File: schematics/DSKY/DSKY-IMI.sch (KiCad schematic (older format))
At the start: 7 parts, among them J103 Conn_02x08, J104 Conn_02x10, U19 74LS04, U42 74LS04, U46 74LS04, U5 74LS04, U6 74LS00

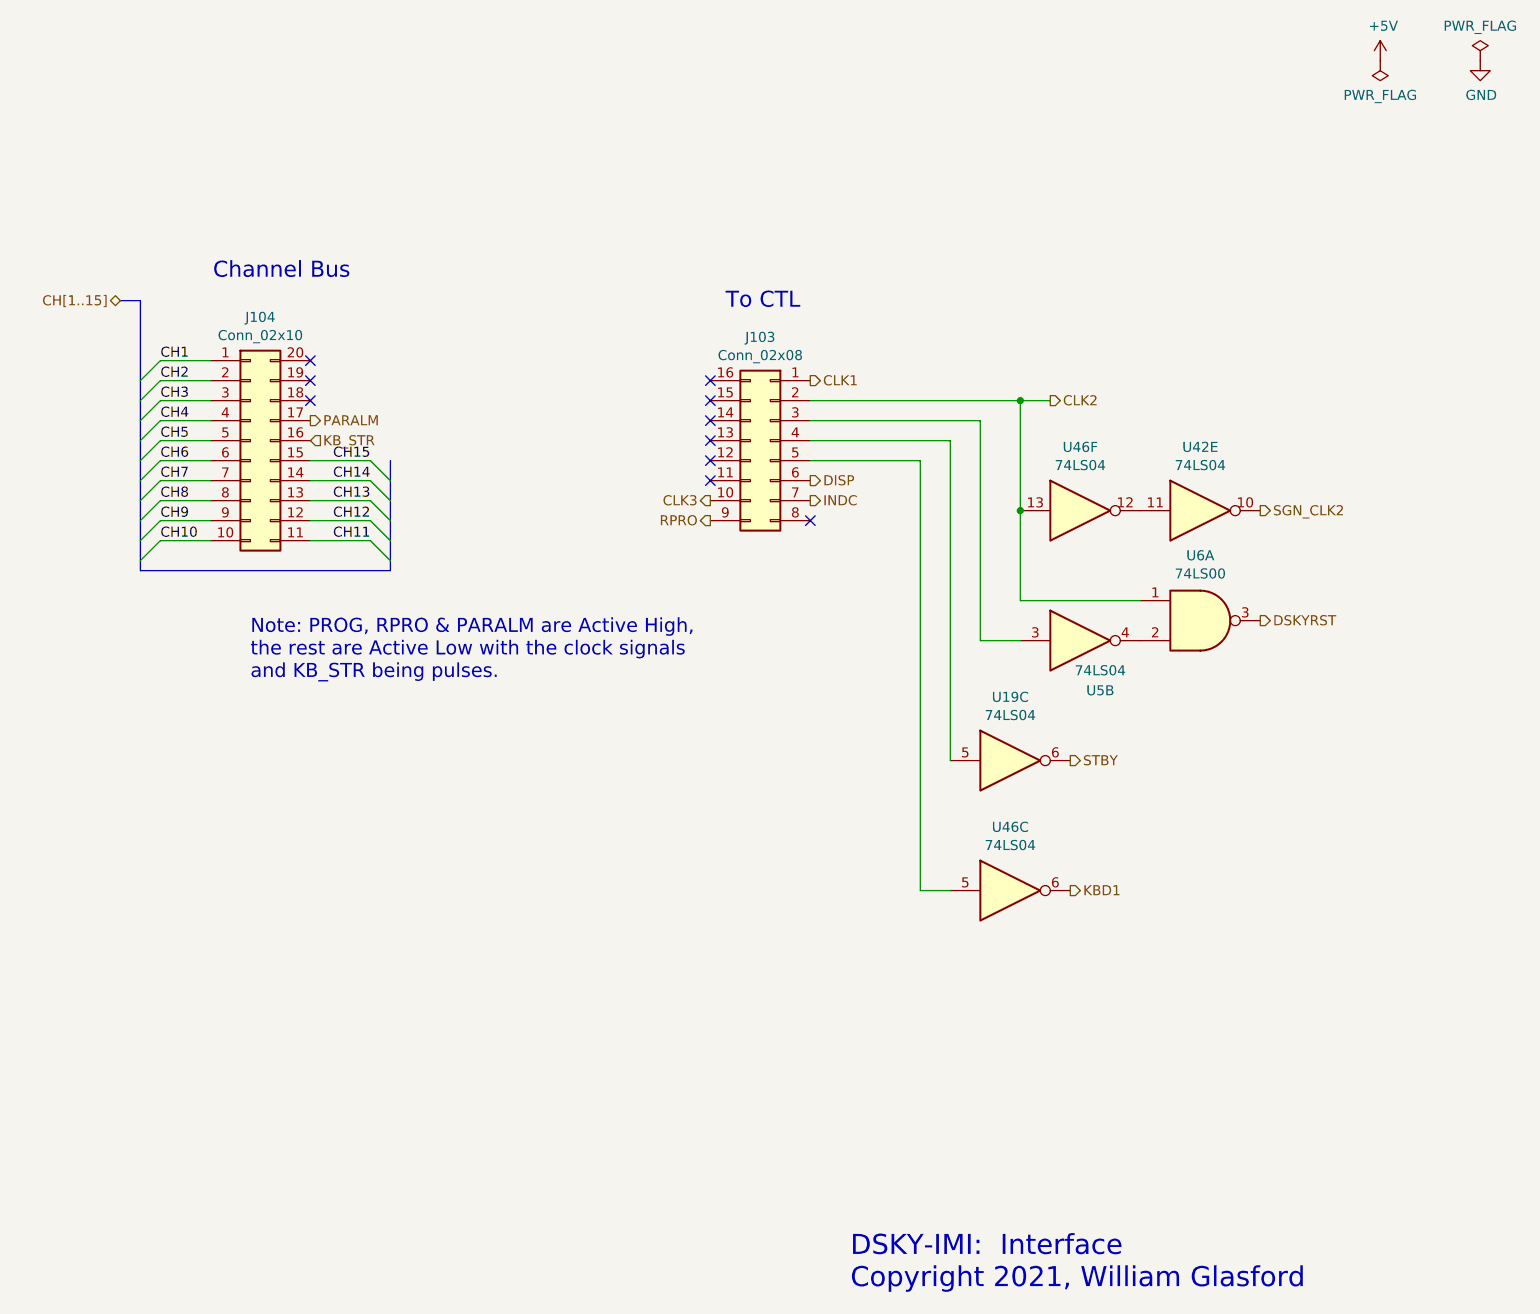
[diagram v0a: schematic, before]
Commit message: DSKY Redesign
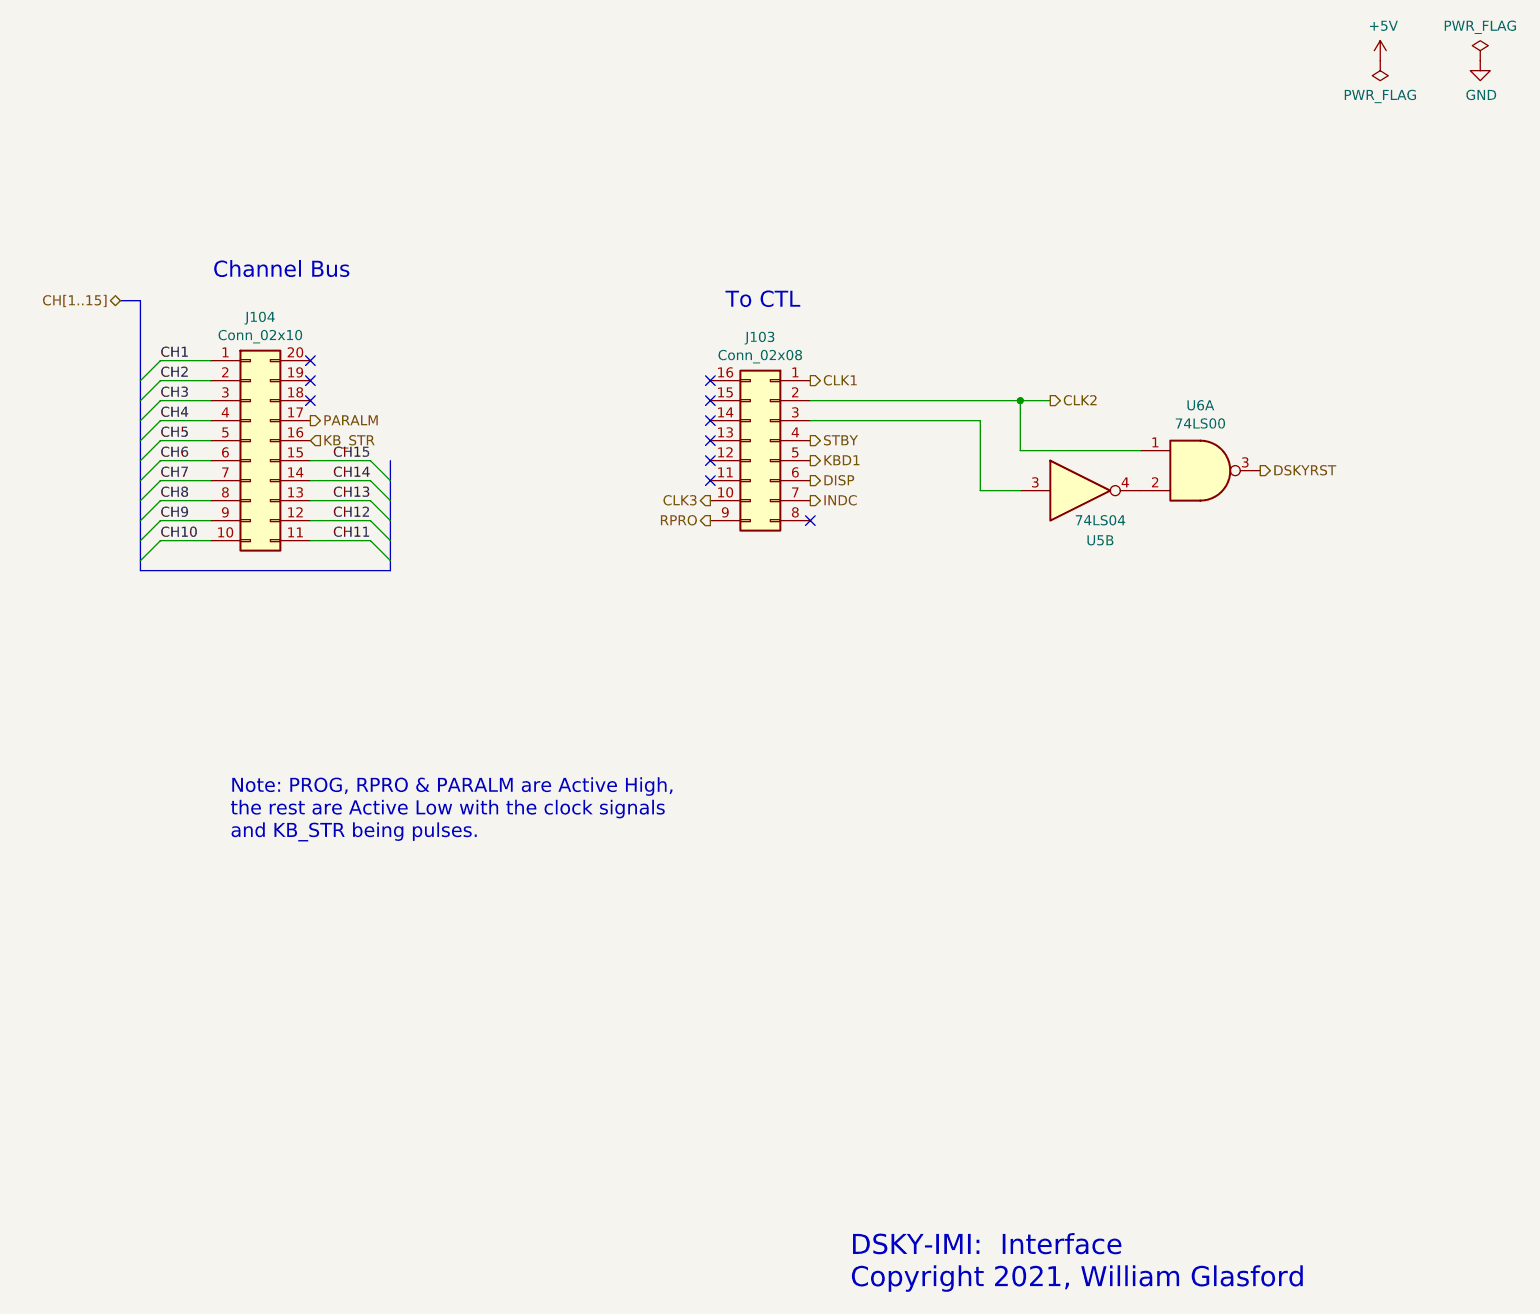
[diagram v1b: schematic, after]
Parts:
- removed U19, U42, U46: 74LS04, symbol 74xx:74LS04
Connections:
- net KBD1: now also J103.5 (Pin_5)
- net STBY: now also J103.4 (Pin_4)
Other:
- moved on the sheet: U5B, U6A
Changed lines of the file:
@@
 $Descr A 11000 8500
 encoding utf-8
-Sheet 10 12
+Sheet 2 15
 Title ""
 Date ""
@@
 Wire Wire Line
 	3750 3000 4050 3000
-Text HLabel 7550 4500 2    50   Output ~ 0
+Text HLabel 6250 2900 2    50   Output ~ 0
 STBY
 Text HLabel 3750 2900 2    50   Input ~ 0
@@
 Text Notes 6200 2250 2    80   ~ 0
 To CTL
-Text HLabel 7550 5150 2    50   Output ~ 0
+Text HLabel 6250 3000 2    50   Output ~ 0
 KBD1
 Text HLabel 6250 3100 2    50   Output ~ 0
@@
 Text HLabel 6250 3200 2    50   Output ~ 0
 INDC
-NoConn ~ 5750 3100
 Text Notes 6450 7150 0    100  ~ 0
 DSKY-IMI:  Interface\nCopyright 2021, William Glasford
@@
 Text HLabel 5750 3300 0    50   Output ~ 0
 RPRO
-Text HLabel 8500 3800 2    50   Output ~ 0
+Text HLabel 8500 3050 2    50   Output ~ 0
 DSKYRST
 $Comp
 L 74xx:74LS00 U?
 U 1 1 6395652F
-P 8200 3800
+P 8200 3050
 AR Path="/5F5E4E3B/5F5F8347/6395652F" Ref="U?"  Part="1"
 AR Path="/60F98A72/6395652F" Ref="U?"  Part="1"
@@
 AR Path="/60F98A72/66CE2F9E/6395652F" Ref="U?"  Part="1"
 AR Path="/60F989FD/6395652F" Ref="U6"  Part="1"
-F 0 "U6" H 8200 4125 50  0000 C CNN
-F 1 "74LS00" H 8200 4034 50  0000 C CNN
-F 2 "" H 8200 3800 50  0001 C CNN
-F 3 "http://www.ti.com/lit/gpn/sn74ls00" H 8200 3800 50  0001 C CNN
-	1    8200 3800
+F 0 "U6" H 8200 3375 50  0000 C CNN
+F 1 "74LS00" H 8200 3284 50  0000 C CNN
+F 2 "" H 8200 3050 50  0001 C CNN
+F 3 "http://www.ti.com/lit/gpn/sn74ls00" H 8200 3050 50  0001 C CNN
+	1    8200 3050
 	1    0    0    -1
 $EndComp
@@
 L 74xx:74LS04 U?
 U 2 1 63956535
-P 7600 3900
+P 7600 3150
 AR Path="/5F5E4E3B/5F5F8347/63956535" Ref="U?"  Part="6"
 AR Path="/60F98A72/63956535" Ref="U?"  Part="2"
@@
 AR Path="/60F98A72/66CE2F9E/63956535" Ref="U?"  Part="6"
 AR Path="/60F989FD/63956535" Ref="U5"  Part="2"
-F 0 "U5" H 7700 3650 50  0000 C CNN
-F 1 "74LS04" H 7700 3750 50  0000 C CNN
-F 2 "" H 7600 3900 50  0001 C CNN
-F 3 "http://www.ti.com/lit/gpn/sn74LS04" H 7600 3900 50  0001 C CNN
-	2    7600 3900
+F 0 "U5" H 7700 2900 50  0000 C CNN
+F 1 "74LS04" H 7700 3000 50  0000 C CNN
+F 2 "" H 7600 3150 50  0001 C CNN
+F 3 "http://www.ti.com/lit/gpn/sn74LS04" H 7600 3150 50  0001 C CNN
+	2    7600 3150
 	1    0    0    -1
 $EndComp
@@
 	6250 2800 7100 2800
 Wire Wire Line
-	7100 2800 7100 3900
-Wire Wire Line
-	7100 3900 7300 3900
-$Comp
-L 74xx:74LS04 U42
-U 5 1 6247150B
-P 8200 3250
-F 0 "U42" H 8200 3567 50  0000 C CNN
-F 1 "74LS04" H 8200 3476 50  0000 C CNN
-F 2 "" H 8200 3250 50  0001 C CNN
-F 3 "http://www.ti.com/lit/gpn/sn74LS04" H 8200 3250 50  0001 C CNN
-	5    8200 3250
-	1    0    0    -1
-$EndComp
-$Comp
-L 74xx:74LS04 U46
-U 6 1 62471E0E
-P 7600 3250
-F 0 "U46" H 7600 3567 50  0000 C CNN
-F 1 "74LS04" H 7600 3476 50  0000 C CNN
-F 2 "" H 7600 3250 50  0001 C CNN
-F 3 "http://www.ti.com/lit/gpn/sn74LS04" H 7600 3250 50  0001 C CNN
-	6    7600 3250
-	1    0    0    -1
-$EndComp
+	7100 2800 7100 3150
+Wire Wire Line
+	7100 3150 7300 3150
 Wire Wire Line
 	6250 2700 7300 2700
@@
 	7450 2700 7300 2700
 Wire Wire Line
-	7300 3700 7900 3700
-Text HLabel 8500 3250 2    50   Output ~ 0
-SGN_CLK2
-Wire Wire Line
-	7300 2700 7300 3250
-Connection ~ 7300 3250
-Wire Wire Line
-	7300 3250 7300 3700
-Text Notes 3450 4100 0    70   ~ 0
+	7300 2950 7900 2950
+Text Notes 3350 4900 0    70   ~ 0
 Note: PROG, RPRO & PARALM are Active High,\nthe rest are Active Low with the clock signals\nand KB_STR being pulses.
-$Comp
-L 74xx:74LS04 U19
-U 3 1 61EE72FE
-P 7250 4500
-F 0 "U19" H 7250 4817 50  0000 C CNN
-F 1 "74LS04" H 7250 4726 50  0000 C CNN
-F 2 "" H 7250 4500 50  0001 C CNN
-F 3 "http://www.ti.com/lit/gpn/sn74LS04" H 7250 4500 50  0001 C CNN
-	3    7250 4500
-	1    0    0    -1
-$EndComp
-Wire Wire Line
-	6250 2900 6950 2900
-Wire Wire Line
-	6950 2900 6950 4500
-$Comp
-L 74xx:74LS04 U46
-U 3 1 61F122AA
-P 7250 5150
-F 0 "U46" H 7250 5467 50  0000 C CNN
-F 1 "74LS04" H 7250 5376 50  0000 C CNN
-F 2 "" H 7250 5150 50  0001 C CNN
-F 3 "http://www.ti.com/lit/gpn/sn74LS04" H 7250 5150 50  0001 C CNN
-	3    7250 5150
-	1    0    0    -1
-$EndComp
-Wire Wire Line
-	6250 3000 6800 3000
-Wire Wire Line
-	6800 3000 6800 5150
-Wire Wire Line
-	6800 5150 6950 5150
-Text HLabel 5750 3200 0    50   Output ~ 0
-CLK3
 Wire Bus Line
 	2900 3550 4150 3550
 Connection ~ 7300 2700
 NoConn ~ 6250 3300
+Wire Wire Line
+	7300 2700 7300 2950
+NoConn ~ 5750 3100
 Wire Bus Line
 	4150 3000 4150 3550
 Wire Bus Line
 	2900 2200 2900 3550
+Text HLabel 5750 3200 0    50   Output ~ 0
+CLK3
 $EndSCHEMATC
